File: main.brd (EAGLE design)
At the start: 100 x 50 mm, 85 parts, among them IC1 LD1117S50TR, IC2 LD398533RM, IC4 PM8834-SO08N, IC5 PM8834-SO08N, J1 RJ11, Q10 IRF3205SPBF, Q11 IRF3205SPBF, Q12 IRF3205SPBF, Q13 IRF3205SPBF, Q2 BSS138, Q3 BSS138, Q6 BSS138, Q9 BSS138, U1 ESP-WROOM-32, U2 TMP275AIDR, U3 TSL2561T, X1 1751248, X2 1751280, X3 1751277

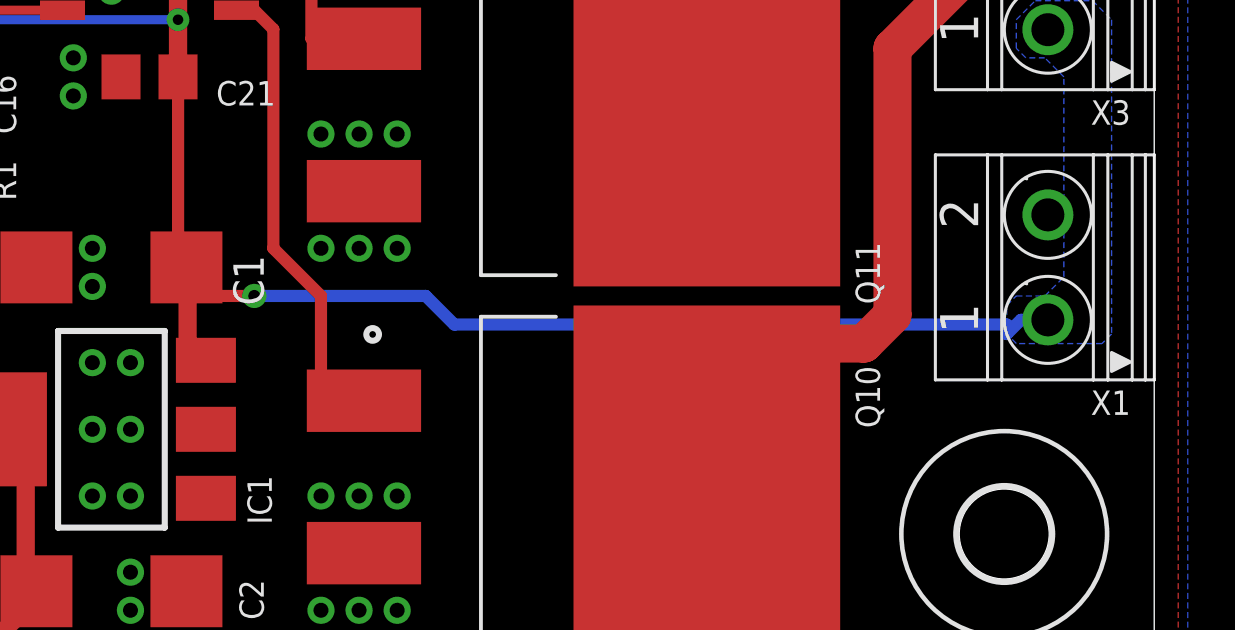
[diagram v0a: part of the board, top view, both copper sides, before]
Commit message: work on programmer board
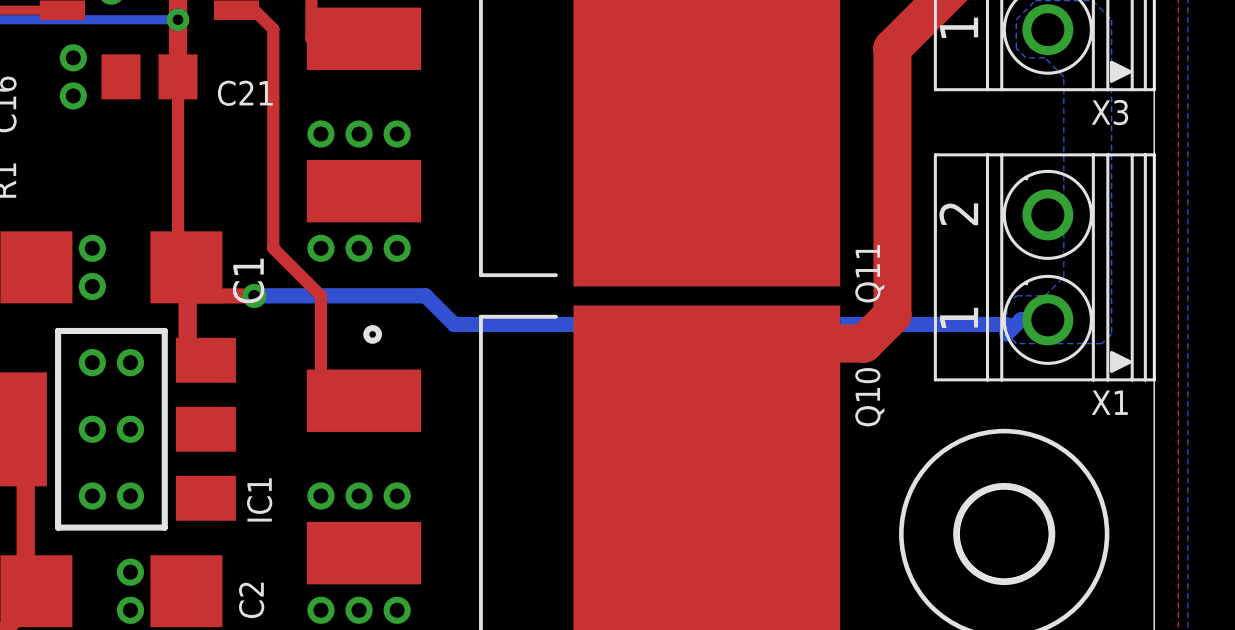
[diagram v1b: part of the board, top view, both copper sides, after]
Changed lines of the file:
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@@
 <wire x1="17.4625" y1="-4.76375" x2="17.4625" y2="-10.835" width="0.4064" layer="1"/>
 <wire x1="17.74" y1="-11.1125" x2="17.4625" y2="-10.835" width="0.4064" layer="1"/>
-<wire x1="46.455" y1="-12.8625" x2="45.5575" y2="-12.8625" width="0.4064" layer="16"/>
-<wire x1="45.5575" y1="-12.8625" x2="45.085" y2="-13.335" width="0.4064" layer="16"/>
+<wire x1="46.455" y1="-12.8625" x2="45.5575" y2="-12.8625" width="0.508" layer="16"/>
+<wire x1="45.5575" y1="-12.8625" x2="45.085" y2="-13.335" width="0.508" layer="16"/>
 <wire x1="45.085" y1="-13.335" x2="45.085" y2="-13.0175" width="0.4064" layer="16"/>
-<wire x1="26.67" y1="-13.0175" x2="25.7175" y2="-12.065" width="0.4064" layer="16"/>
-<wire x1="25.7175" y1="-12.065" x2="20.0025" y2="-12.065" width="0.4064" layer="16"/>
-<wire x1="45.085" y1="-13.0175" x2="26.67" y2="-13.0175" width="0.4064" layer="16"/>
+<wire x1="26.67" y1="-13.0175" x2="25.7175" y2="-12.065" width="0.508" layer="16"/>
+<wire x1="25.7175" y1="-12.065" x2="20.0025" y2="-12.065" width="0.508" layer="16"/>
+<wire x1="45.085" y1="-13.0175" x2="26.67" y2="-13.0175" width="0.508" layer="16"/>
 <via x="20.0025" y="-12.065" extent="1-16" drill="0.4"/>
-<wire x1="20.0025" y1="-12.065" x2="17.78" y2="-12.065" width="0.4064" layer="1"/>
+<wire x1="20.0025" y1="-12.065" x2="17.78" y2="-12.065" width="0.508" layer="1"/>
 <wire x1="7.305" y1="-2.855" x2="7.3025" y2="-2.8575" width="0.3048" layer="1"/>
 <via x="7.3025" y="-2.8575" extent="1-16" drill="0.35"/>
